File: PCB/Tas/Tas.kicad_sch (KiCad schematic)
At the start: 34 parts, among them J1 Shelly 1, J2 Conn_01x07, J3 USB-C-Socket-V, Q1 PMF170XP,115, Q2 PMF250XNEX, U1 FT231XQ, U3 MD8942

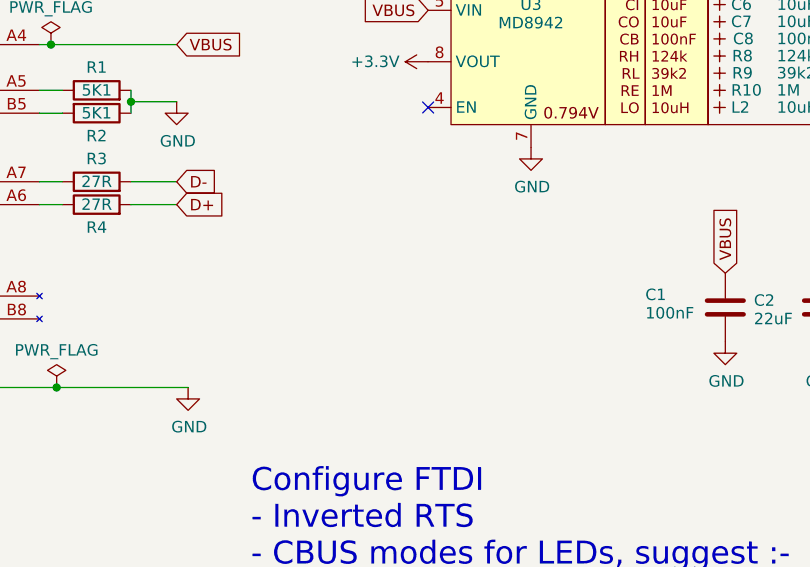
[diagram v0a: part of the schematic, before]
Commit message: As ordered
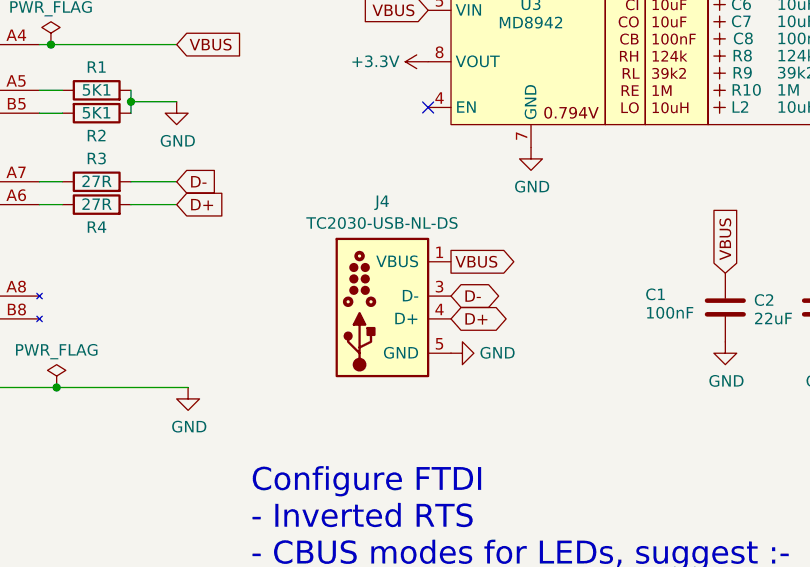
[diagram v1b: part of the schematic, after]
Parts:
- added J4: TC2030-USB-NL-DS, RevK:Tag-Connect_TC2030-IDC-NL_2x03_P1.27mm_Vertical, symbol RevK:TC2030-USB-NL
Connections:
- net D+: now also J4.4 (D+)
- net D-: now also J4.3 (D-)
- net GND: now also J4.5 (GND), J4.6 (GND)
- net VBUS: now also J4.1 (VBUS), J4.2 (VBUS)
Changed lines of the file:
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@@
 		)
 	)
+	(global_label "D+"
+		(shape bidirectional)
+		(at 199.39 76.2 0)
+		(fields_autoplaced yes)
+		(effects
+			(font
+				(size 1.27 1.27)
+			)
+			(justify left)
+		)
+		(property "Intersheetrefs" "${INTERSHEET_REFS}"
+			(at 205.5159 76.2 0)
+			(effects
+				(font
+					(size 1.27 1.27)
+				)
+				(justify left)
+				(hide yes)
+			)
+		)
+	)
 	(global_label "GPIO0"
 		(shape output)
@@
 		)
 	)
+	(global_label "D-"
+		(shape bidirectional)
+		(at 199.39 73.66 0)
+		(fields_autoplaced yes)
+		(effects
+			(font
+				(size 1.27 1.27)
+			)
+			(justify left)
+		)
+		(property "Intersheetrefs" "${INTERSHEET_REFS}"
+			(at 205.5159 73.66 0)
+			(effects
+				(font
+					(size 1.27 1.27)
+				)
+				(justify left)
+				(hide yes)
+			)
+		)
+	)
 	(global_label "RXD"
 		(shape input)
@@
 		)
 	)
+	(global_label "VBUS"
+		(shape output)
+		(at 199.39 69.85 0)
+		(fields_autoplaced yes)
+		(effects
+			(font
+				(size 1.27 1.27)
+			)
+			(justify left)
+		)
+		(property "Intersheetrefs" "${INTERSHEET_REFS}"
+			(at 206.6196 69.85 0)
+			(effects
+				(font
+					(size 1.27 1.27)
+				)
+				(justify left)
+				(hide yes)
+			)
+		)
+	)
 	(global_label "RXD"
 		(shape input)
@@
 	)
 	(symbol
+		(lib_id "power:GND")
+		(at 199.39 80.01 90)
+		(unit 1)
+		(exclude_from_sim no)
+		(in_bom yes)
+		(on_board yes)
+		(dnp no)
+		(fields_autoplaced yes)
+		(property "Reference" "#PWR010"
+			(at 205.74 80.01 0)
+			(effects
+				(font
+					(size 1.27 1.27)
+				)
+				(hide yes)
+			)
+		)
+		(property "Value" "GND"
+			(at 202.565 80.01 90)
+			(effects
+				(font
+					(size 1.27 1.27)
+				)
+				(justify right)
+			)
+		)
+		(property "Footprint" ""
+			(at 199.39 80.01 0)
+			(effects
+				(font
+					(size 1.27 1.27)
+				)
+				(hide yes)
+			)
+		)
+		(property "Datasheet" ""
+			(at 199.39 80.01 0)
+			(effects
+				(font
+					(size 1.27 1.27)
+				)
+				(hide yes)
+			)
+		)
+		(property "Description" "Power symbol creates a global label with name \"GND\" , ground"
+			(at 199.39 80.01 0)
+			(effects
+				(font
+					(size 1.27 1.27)
+				)
+				(hide yes)
+			)
+		)
+		(pin "1"
+		)
+		(instances
+			(project "Tas"
+				(path "/42713045-fffd-4b2d-ae1e-7232d705fb12"
+					(reference "#PWR010")
+					(unit 1)
+				)
+			)
+		)
+	)
+	(symbol
 		(lib_id "Device:R")
 		(at 181.61 144.145 270)
@@
 					(unit 1)
 				)
+			)
+		)
+	)
+	(symbol
+		(lib_id "RevK:TC2030-USB-NL")
+		(at 191.77 74.93 0)
+		(unit 1)
+		(exclude_from_sim no)
+		(in_bom no)
+		(on_board yes)
+		(dnp no)
+		(fields_autoplaced yes)
+		(property "Reference" "J4"
+			(at 191.77 63.1655 0)
+			(effects
+				(font
+					(size 1.27 1.27)
+				)
+			)
+		)
+		(property "Value" "TC2030-USB-NL-DS"
+			(at 191.77 65.5898 0)
+			(effects
+				(font
+					(size 1.27 1.27)
+				)
+			)
+		)
+		(property "Footprint" "RevK:Tag-Connect_TC2030-IDC-NL_2x03_P1.27mm_Vertical"
+			(at 191.516 84.074 0)
+			(effects
+				(font
+					(size 1.27 1.27)
+				)
+				(hide yes)
+			)
+		)
+		(property "Datasheet" " ~"
+			(at 195.58 76.2 0)
+			(effects
+				(font
+					(size 1.27 1.27)
+				)
+				(hide yes)
+			)
+		)
+		(property "Description" "TC2030-USB-NL"
+			(at 191.77 62.23 0)
+			(effects
+				(font
+					(size 1.27 1.27)
+				)
+				(hide yes)
+			)
+		)
+		(pin "5"
+		)
+		(pin "6"
+		)
+		(pin "1"
+		)
+		(pin "4"
+		)
+		(pin "3"
+		)
+		(pin "2"
+		)
+		(instances
+			(project "Tas"
+				(path "/42713045-fffd-4b2d-ae1e-7232d705fb12"
+					(reference "J4")
+					(unit 1)
+				)
